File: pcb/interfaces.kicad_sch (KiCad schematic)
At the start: 22 parts, among them J10 BM08B-SRSS-TB, J14 BM03B-SRSS-TB, J3 BM03B-SRSS-TB, J8 BM04B-SRSS-TB, J9 BM04B-SRSS-TB, Q1 MMBT2222A

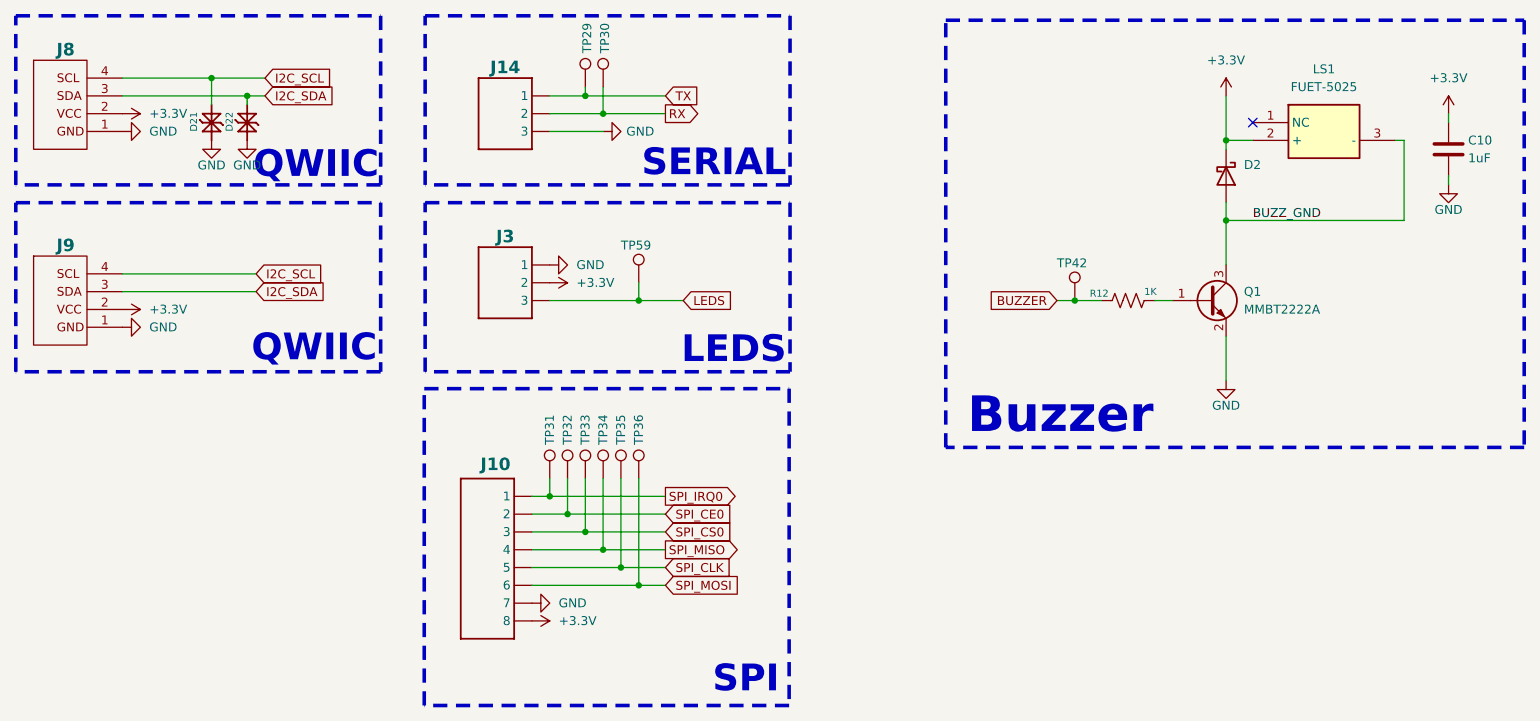
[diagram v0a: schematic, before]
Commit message: Clean up and consistency
Moved buzzer to MCU
Fixed model directory
Set font size
Set outline size
Upscaled Roxy ❤️
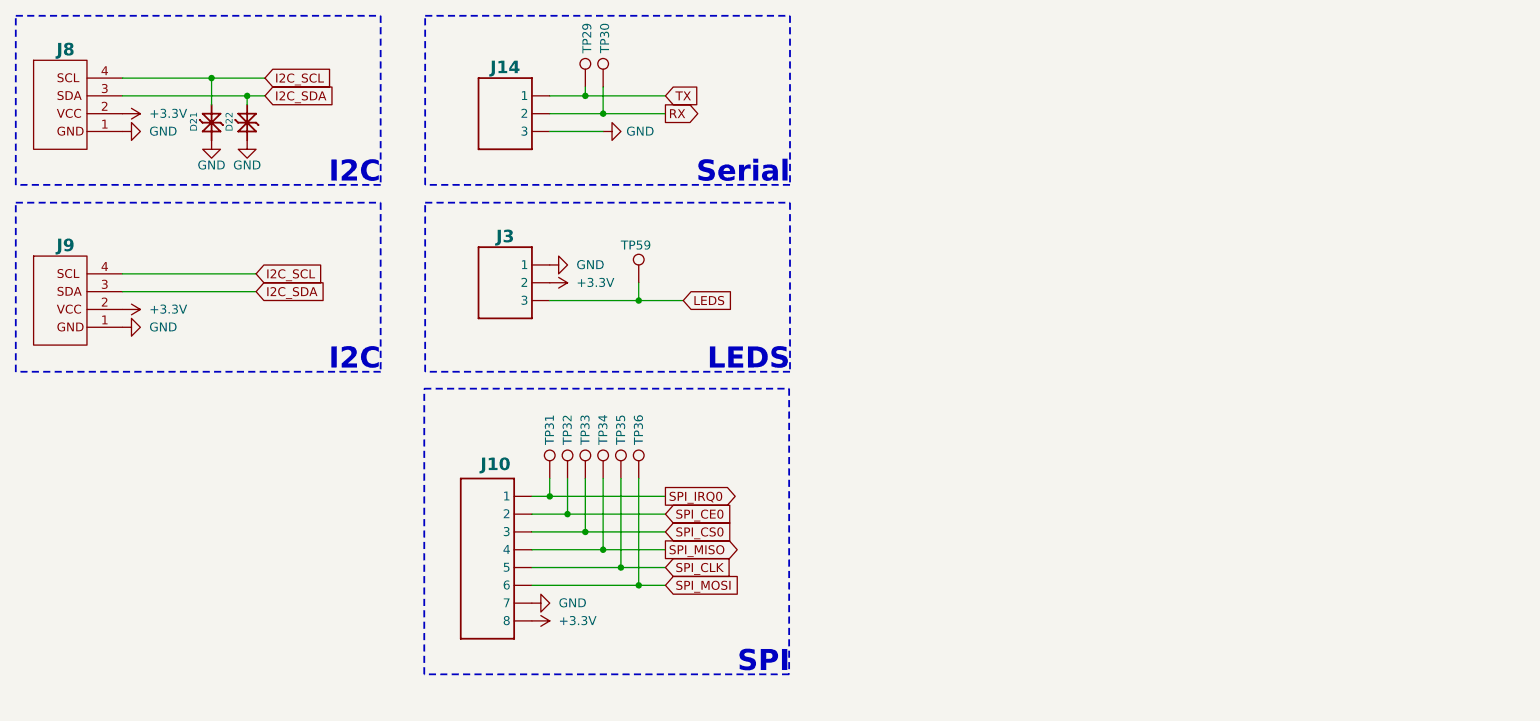
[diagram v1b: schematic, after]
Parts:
- removed C10: 1uF, CRGM Passive:C_0603_1608Metric, symbol Device:C
- removed D2: D_Schottky, CRGM Passive:D_SOD-523, symbol Device:D_Schottky
- removed LS1: FUET-5025, CRG Makes:FUET-5025, symbol CRG Makes:CMT-0502-75-SMT-TR
- removed Q1: MMBT2222A, CRGM Passive:SOT-523, symbol Transistor_BJT:MMBT2222A
- removed R12: 1K, CRGM Passive:R_0603_1608Metric, symbol Device:R_US
- removed TP42: ~, CRGM Mechanical:TestPoint_Pad_D1.0mm, symbol Connector:TestPoint
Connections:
- no-connect marks 1 -> 0
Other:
- note added: "I2C"
- note added: "Serial"
- note removed: "Buzzer"
- note removed: "QWIIC"
- note removed: "SERIAL"
